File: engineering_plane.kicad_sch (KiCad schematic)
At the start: 3 parts, among them U1 TPS54302DDCR, U2 TPS54302DDCR

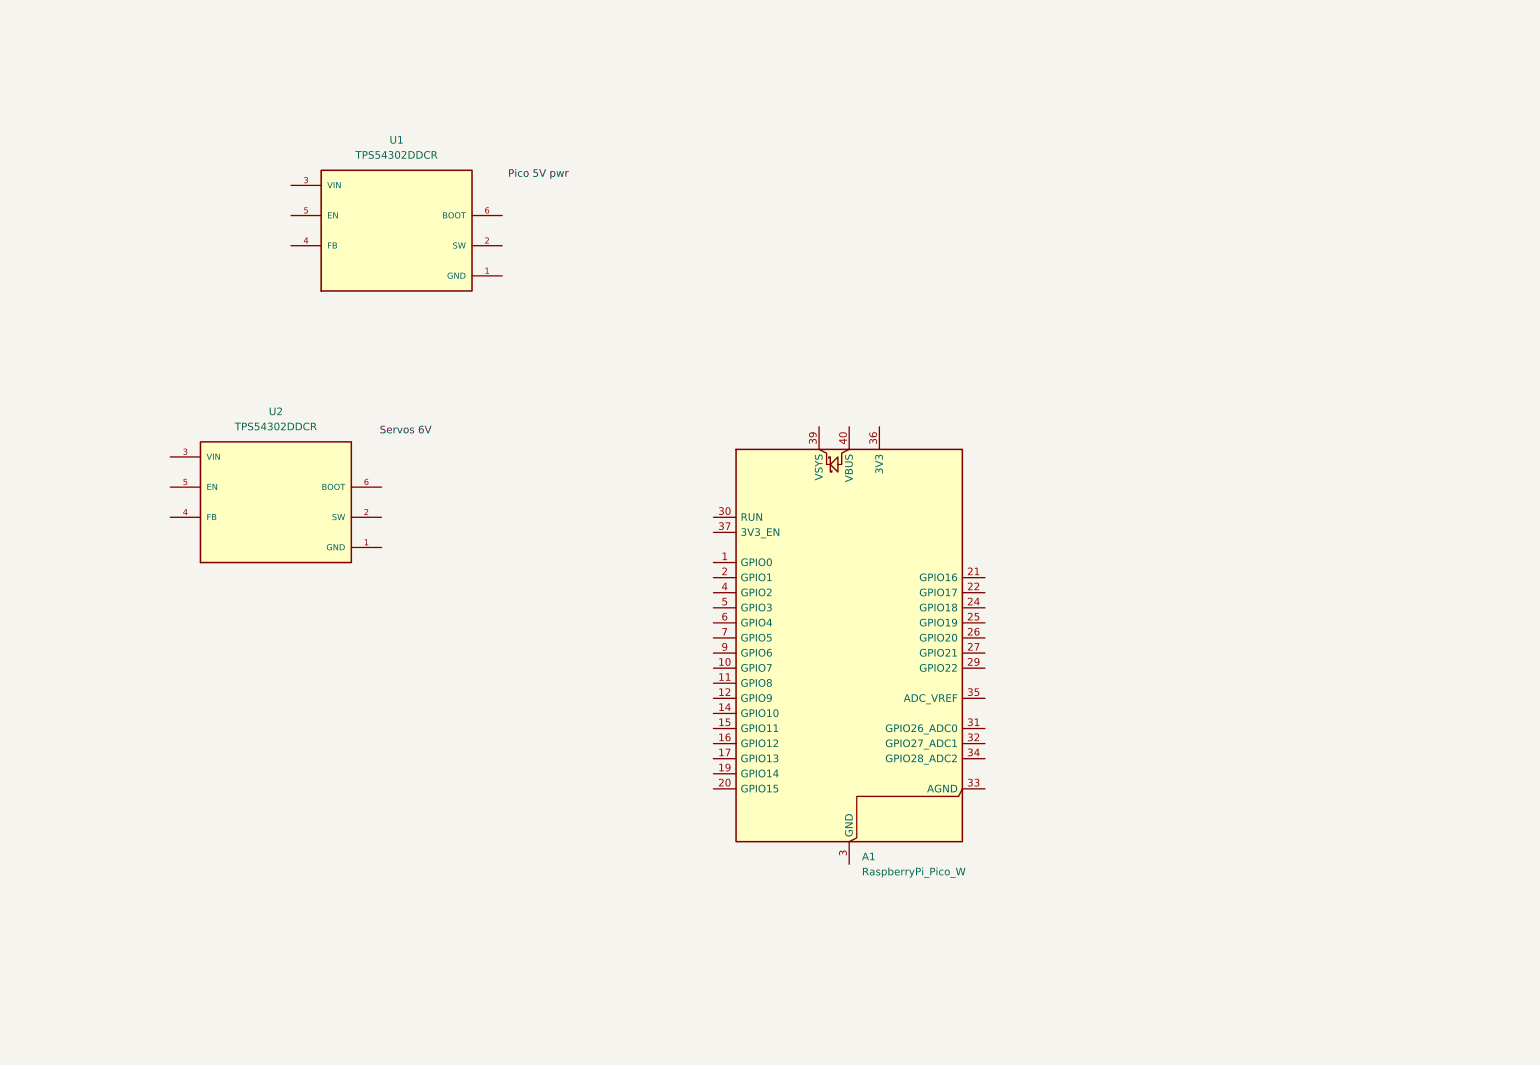
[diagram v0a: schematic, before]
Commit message: feat: power section done, onto sensors
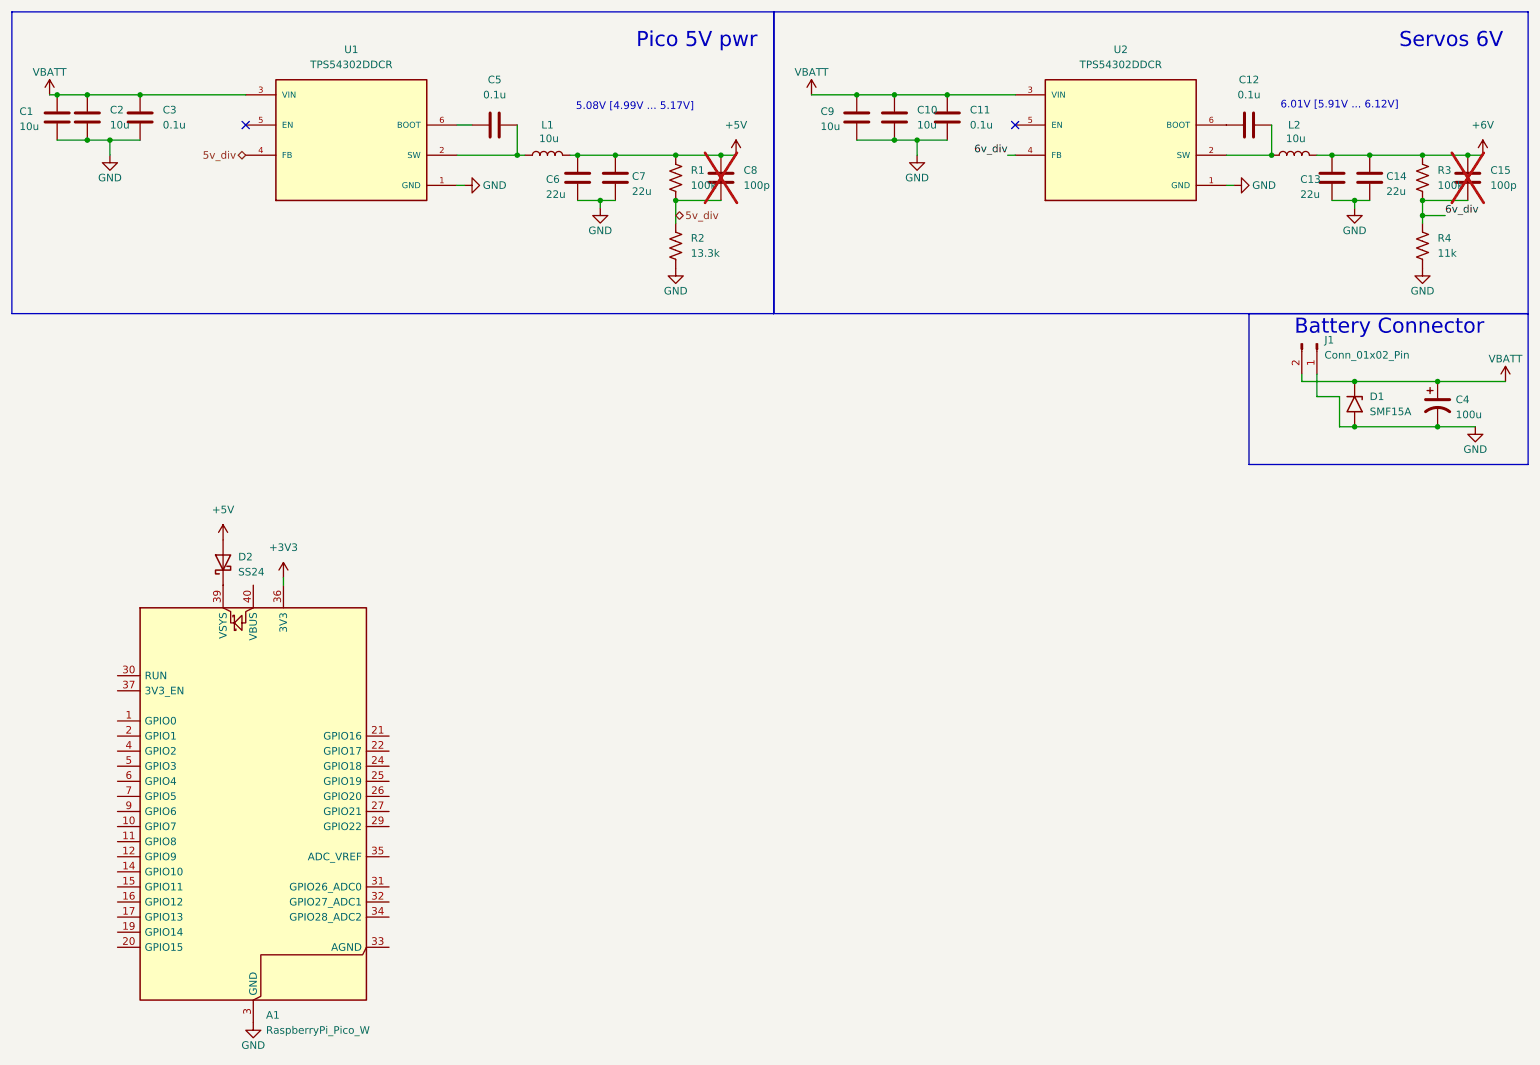
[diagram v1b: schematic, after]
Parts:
- added C1, C10, C2, C9: 10u, Capacitor_SMD:C_1206_3216Metric, symbol Device:C
- added C11, C12, C3, C5: 0.1u, Capacitor_SMD:C_0805_2012Metric, symbol Device:C
- added C13, C14, C6, C7: 22u, Capacitor_SMD:C_1206_3216Metric, symbol Device:C
- added C15, C8: 100p, Capacitor_SMD:C_0805_2012Metric, symbol Device:C
- added C4: 100u, Capacitor_SMD:CP_Elec_6.3x7.7, symbol PCM_SparkFun-Capacitor:C_Polarized
- added D1: SMF15A, Diode_SMD:D_SMF, symbol Diode:SMF15A
- added D2: SS24, Diode_SMD:D_SMA, symbol Diode:SS24
- added J1: Conn_01x02_Pin, Connector_AMASS:AMASS_XT30PW-M_1x02_P2.50mm_Horizontal, symbol Connector:Conn_01x02_Pin
- added L1, L2: 10u, Inductor_SMD:L_7.3x7.3_H4.5, symbol Device:L
- added R1, R3: 100k, PCM_SparkFun-Resistor:R_0603_1608Metric, symbol PCM_SparkFun-Resistor:R
- added R2: 13.3k, PCM_SparkFun-Resistor:R_0603_1608Metric, symbol PCM_SparkFun-Resistor:R
- added R4: 11k, PCM_SparkFun-Resistor:R_0603_1608Metric, symbol PCM_SparkFun-Resistor:R
- U1, U2: footprint TPS54302DDCR:SOT95P280X110-6N -> TPS54302:SOT95P280X110-6N
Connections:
- net GND: now reaches U2.1 (GND)
- net GND: now also A1.13 (GND), A1.18 (GND), A1.23 (GND), A1.28 (GND), A1.3 (GND), A1.38 (GND), A1.8 (GND), U1.1 (GND), C1.2, C10.2, C11.2, C13.2, C14.2, C2.2, C3.2, C4.2, C6.2, C7.2, C9.2, D1.2 (A2), J1.1 (Pin_1), R2.1, R4.1
- net at U2.2 (SW): now also C12.2, L2.1
- net VBATT: now reaches U2.3 (VIN)
- net VBATT: now also U1.3 (VIN), C1.1, C10.1, C11.1, C2.1, C3.1, C4.1, C9.1, D1.1 (A1), J1.2 (Pin_2)
- net 6v_div: now reaches U2.4 (FB)
- net 6v_div: now also C15.2, R3.1, R4.2
- net at U2.6 (BOOT): now also C12.1
- net +3V3: now reaches A1.36 (3V3)
- net at A1.39 (VSYS): now also D2.1 (K)
- net at U1.2 (SW): now also C5.2, L1.1
- net 5v_div: now reaches U1.4 (FB)
- net 5v_div: now also C8.2, R1.1, R2.2
- net at U1.6 (BOOT): now also C5.1
- new net +5V: C6.1, C7.1, C8.1, D2.2 (A), L1.2, R1.2
- new net +6V: C13.1, C14.1, C15.1, L2.2, R3.2
- no-connect marks 0 -> 2
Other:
- note added: "5.08V [4.99V ... 5.17V]"
- note added: "6.01V [5.91V ... 6.12V]"
- note added: "Battery Connector"
- moved on the sheet: A1, U1, U2
